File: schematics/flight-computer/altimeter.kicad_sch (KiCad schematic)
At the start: 11 parts, among them U201 TXS0108EPW, U202 ICM-20789, U203 MS5611-01BA

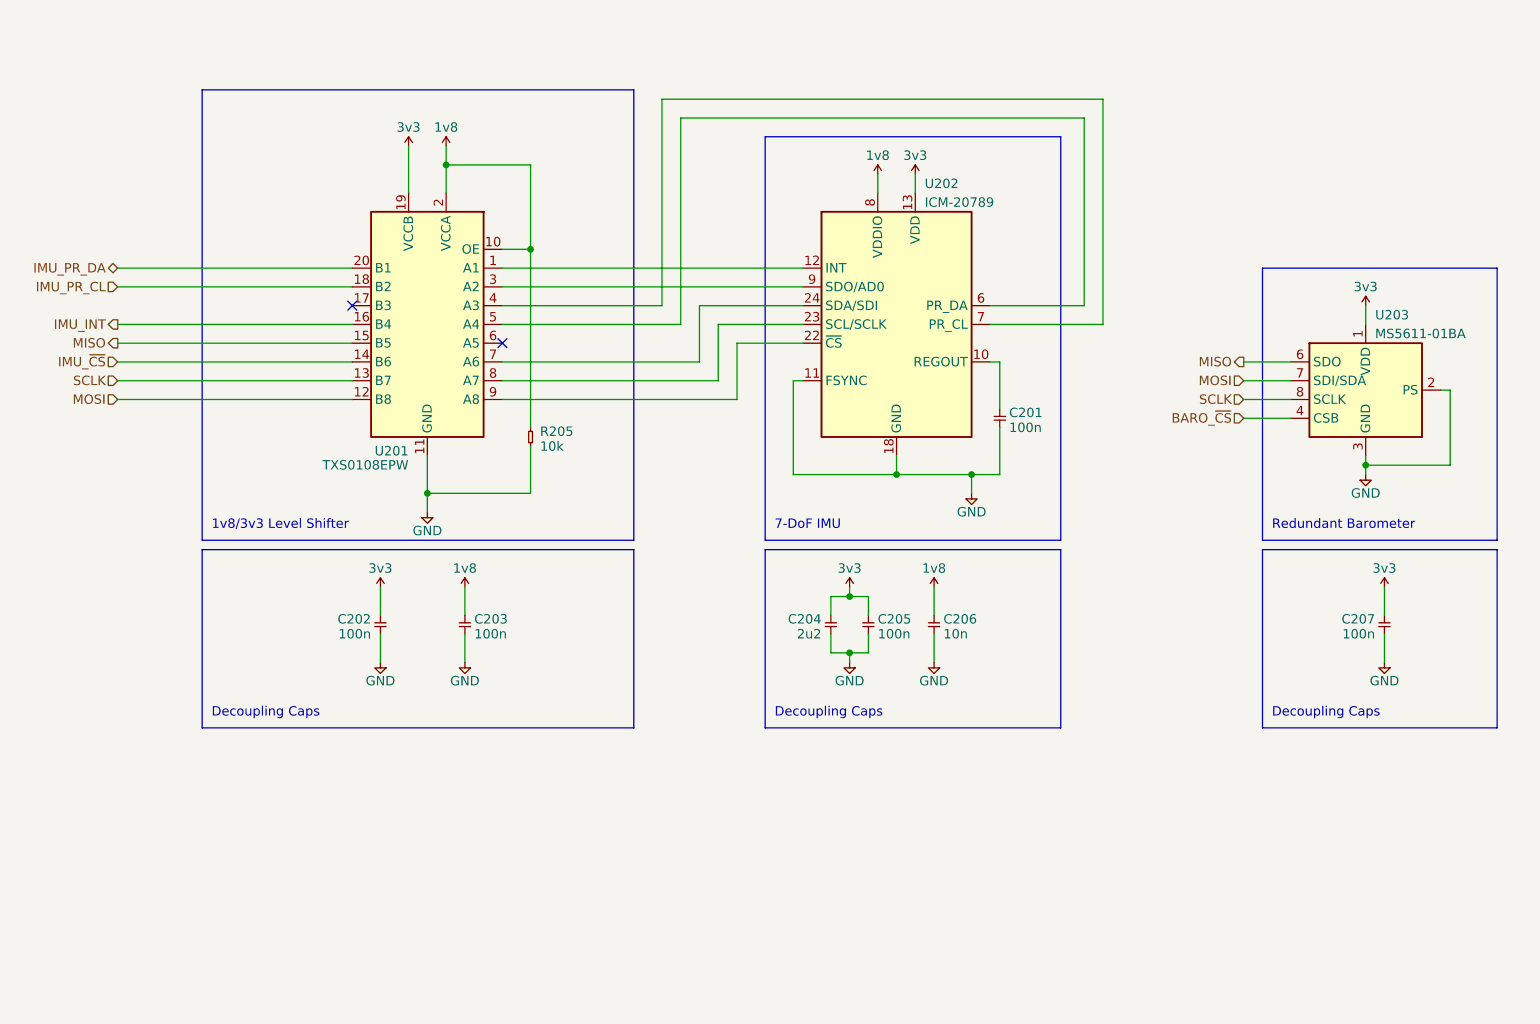
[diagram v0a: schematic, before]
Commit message: Complete first draft
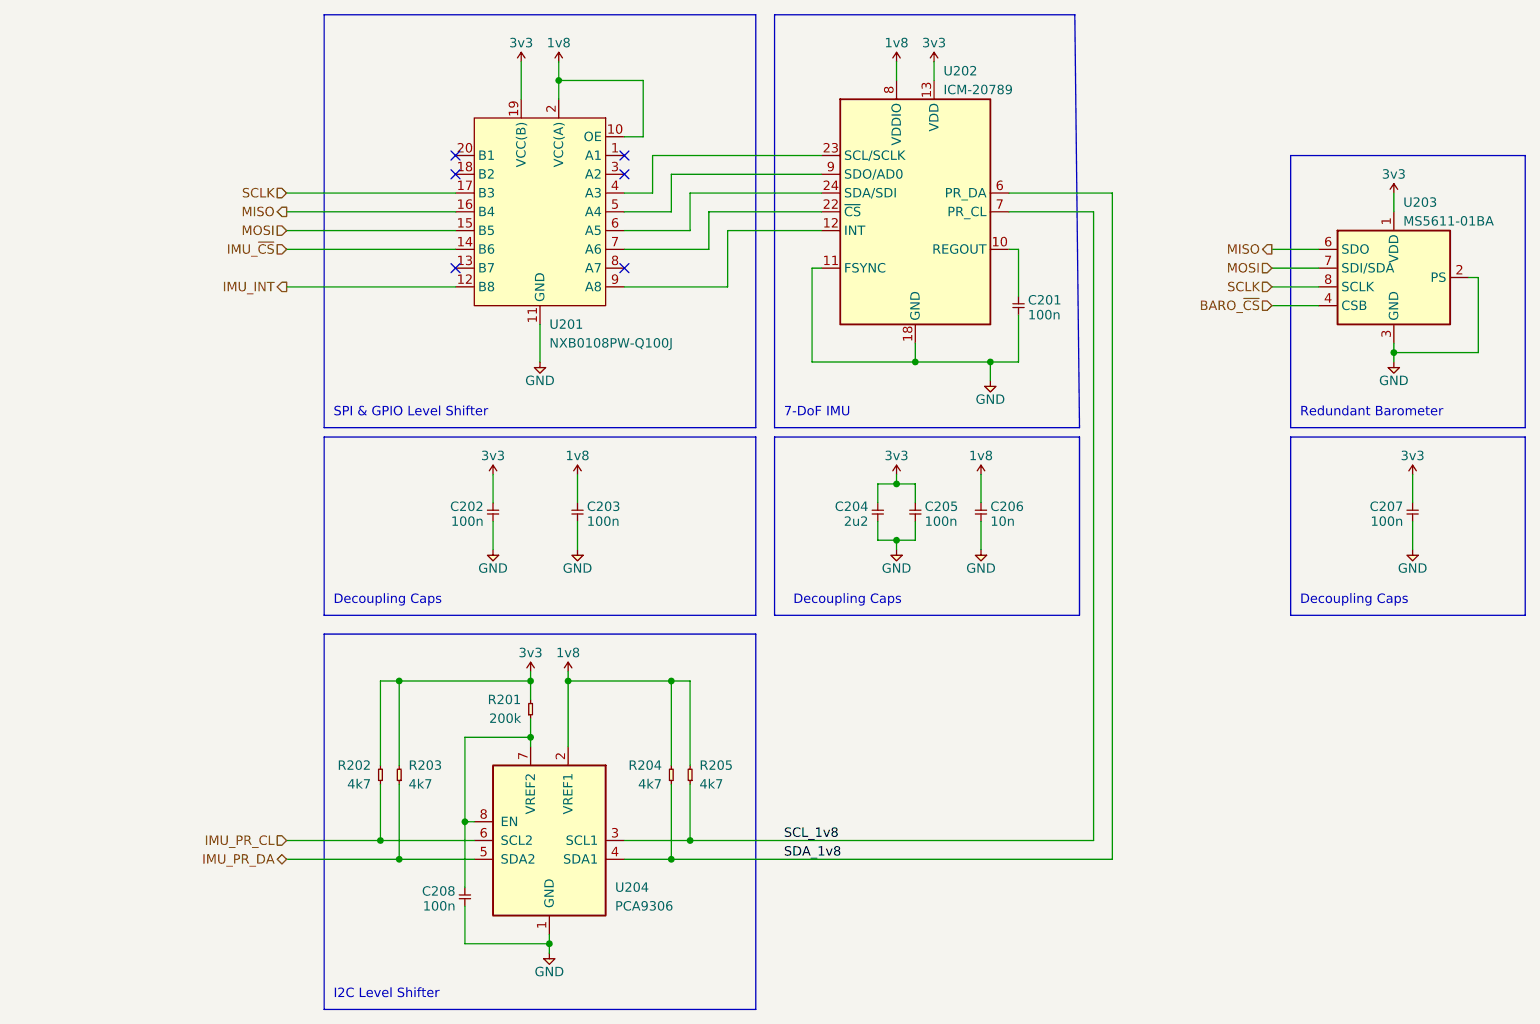
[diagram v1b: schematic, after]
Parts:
- removed U201: TXS0108EPW, Strix:TXS0108EPW, symbol Strix:TXS0108EPW
- added C203: 100n, Strix:C_0402, symbol Strix:C
- added R201: 200k, Strix:R_0402, symbol Strix:R
- added R202, R203, R204: 4k7, Strix:R_0402, symbol Strix:R
- added U201: NXB0108PW-Q100J, Strix:NXB0108PW-Q100J, symbol Strix:NXB0108PW-Q100J
- added U204: PCA9306, Strix:PCA9306, symbol Strix:PCA9306
- C201, C205, C207: Farnell (none) -> 9402047
- C204: Farnell (none) -> 2672111
- C206: Farnell (none) -> 1758924
- R205: value 10k -> 4k7
- renumbered C203 to C208
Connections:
- net 1v8: now also C203.2, R204.2, U201.10 (OE), U201.2 (VCC(A)), U204.2 (VREF1); no longer C208.2
- net 3v3: now also R201.2, R202.2, R203.2, U201.19 (VCC(B))
- net GND: now also C203.1, U201.11 (GND), U204.1 (GND); no longer R205.1
- net IMU_INT: now also U201.12 (B8)
- net IMU_PR_CL: now also R202.1, U204.6 (SCL2)
- net IMU_PR_DA: now also R203.1, U204.5 (SDA2)
- net IMU_~{CS}: now also U201.14 (B6)
- net MISO: now also U201.16 (B4)
- net MOSI: now also U201.15 (B5)
- net SCLK: now also U201.17 (B3)
- net at U202.12 (INT): now also U201.9 (A8)
- net at U202.22 (~{CS}): now also U201.7 (A6)
- net at U202.23 (SCL/SCLK): now also U201.4 (A3)
- net at U202.24 (SDA/SDI): now also U201.6 (A5)
- net SDA_1v8: now reaches U202.6 (PR_DA)
- net SDA_1v8: now also R204.1, U204.4 (SDA1)
- net SCL_1v8: now reaches U202.7 (PR_CL)
- net SCL_1v8: now also R205.1, U204.3 (SCL1)
- net at U202.9 (SDO/AD0): now also U201.5 (A4)
- new net: C208.2, R201.1, U204.7 (VREF2), U204.8 (EN)
- no-connect marks 2 -> 6
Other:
- note added: "I2C Level Shifter"
- note added: "SPI & GPIO Level Shifter"
- note removed: "1v8/3v3 Level Shifter"
- moved on the sheet: C201, C204, C205, C206, C207, C208, U202, U203
